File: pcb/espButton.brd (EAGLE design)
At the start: 23.8 x 49.5 mm, 15 parts, among them CN2 JSTPH, U1 MCP73831T-2ACI/OT

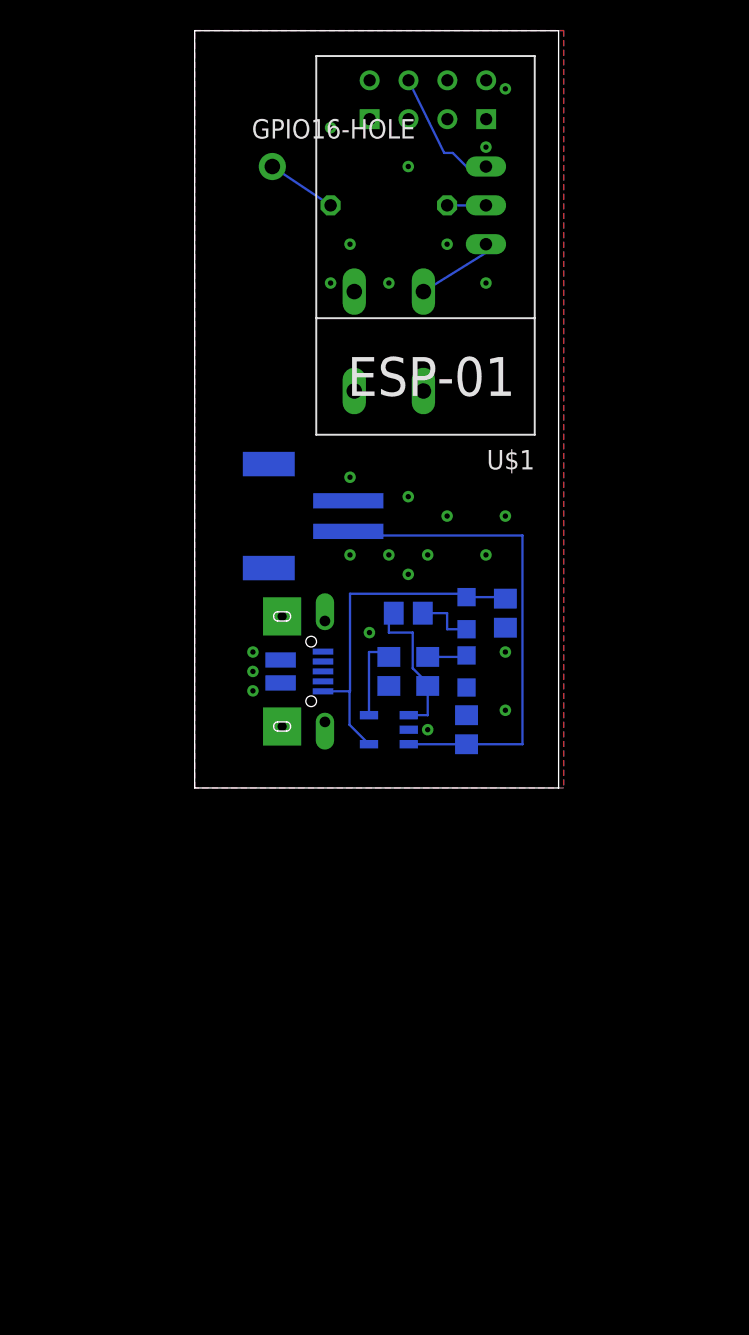
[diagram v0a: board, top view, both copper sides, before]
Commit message: Improved pcb design
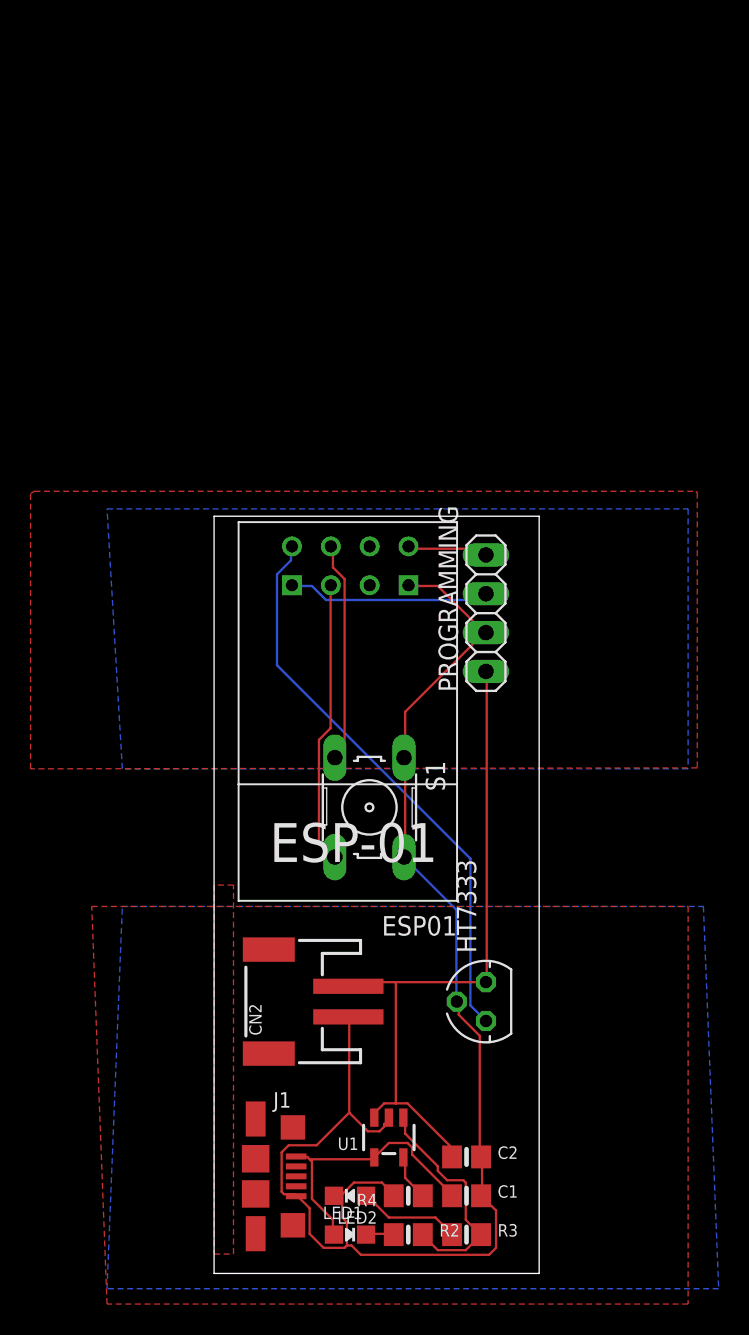
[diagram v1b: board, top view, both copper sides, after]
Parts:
- removed GPIO16-HOLE: (no value), adafruit:1X01-CLEANBIG
- removed R1: 330k, eagle-ltspice:0204/7
- removed T1: (no value), transistor-neu-to92:TO92-EBC
- removed U$1: ESP01, esp8266modules:ESP01
- removed X1: (no value), microbuilder:4UCONN_20329
- added ESP01: ESP01, esp8266modules:ESP01
- added HT7333: (no value), DC_LOAD_AU:78LXX
- added J1: 1981584-1, audio amplifier example:1981584-1
- added PROGRAMMING: (no value), DC_LOAD_AU:1X04
- moved LED1 41.3 mm to (8.89, 2.54), flipped to the top, turned to 270 degrees
- moved R2 40.6 mm to (12.7, 2.54), flipped to the top
- moved C1 38.2 mm to (16.5, 5.08), flipped to the top, turned to 0 degrees
- moved R3 36.9 mm to (16.5, 2.54), flipped to the top, turned to 0 degrees
- moved LED2 35.1 mm to (8.89, 5.08), flipped to the top, turned to 90 degrees
- moved R4 34.3 mm to (12.7, 5.08), flipped to the top, turned to 180 degrees
- moved CN2 31.8 mm to (5.08, 17.8), flipped to the top, turned to 90 degrees
- moved S1 30.5 mm to (10.2, 30.5), flipped to the top
- moved C2 27.9 mm to (16.5, 7.62), flipped to the top, turned to 0 degrees
- moved U1 26.7 mm to (11.4, 8.89), flipped to the top, turned to 180 degrees
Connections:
- removed net GPIO16: GPIO16-HOLE.1, R1.2
- removed net N$2: T1.C, U$1.RST
- removed net VBAT1: C2.1, CN2.2, U1.3
- removed net VDD1: C1.1, LED1.A, U1.4, X1.VBUS
- new net 3V3: ESP01.VCC, HT7333.OUT
- new net BAT: C2.1, CN2.2, HT7333.IN, PROGRAMMING.1, U1.3
- new net PRGM: ESP01.GPIO0, S1.4
- new net RX: ESP01.TX, PROGRAMMING.4
- new net TX: ESP01.RX, PROGRAMMING.3
- net GND: now also ESP01.GND, HT7333.GND, J1.5, PROGRAMMING.2, S1.2; no longer U$1.GND, X1.BASE@1, X1.BASE@2, X1.GND, X1.SPRT@1, X1.SPRT@2, X1.SPRT@3, X1.SPRT@4
- net N$1: now also C1.1, J1.1, LED1.A, U1.4; no longer R1.1, T1.B
- net N$4: now also ESP01.RST; no longer T1.E
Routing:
- net GND: track 0.00 -> 95.3 mm, vias 25 -> 0
- net BAT: track 0.00 -> 44.9 mm
- net 3V3: track 0.00 -> 37.1 mm
- net VBAT1: track 32.6 -> 0.00 mm
- net VDD1: track 22.6 -> 0.00 mm
- net PRGM: track 0.00 -> 18.6 mm
- net N$1: track 2.54 -> 18.0 mm
- net TX: track 0.00 -> 13.2 mm
- net N$4: track 5.37 -> 14.4 mm
- net N$2: track 8.39 -> 0.00 mm
- net RX: track 0.00 -> 5.32 mm
- net N$6: track 10.2 -> 15.1 mm
- net GPIO16: track 4.58 -> 0.00 mm
- net N$8: track 2.64 -> 6.68 mm
- net N$7: track 5.75 -> 3.03 mm
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- added copper zone on layer 1, net N$2
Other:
- board size 23.8 x 49.5 mm -> 21.3 x 49.5 mm
- board text added: "GND"
- board text added: "RX"
- board text added: "TX"
- board text added: "VCC"
- board text removed: "ESPBUTTON"
- board text removed: "Kevin van den Broek"
